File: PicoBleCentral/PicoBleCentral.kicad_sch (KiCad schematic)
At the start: 25 parts, among them J1 Screw_Terminal_01x02, J2 3V3 Sel, J3 keypad, J4 grove 2mm, J5 i2c, Q1 DMG2305UX-7, SW1 SW_Push, U1 AP7384-50Y, U2 Pico_RaspberryPico, U3 MCP23008-xSO, U4 AMS1117-3.3

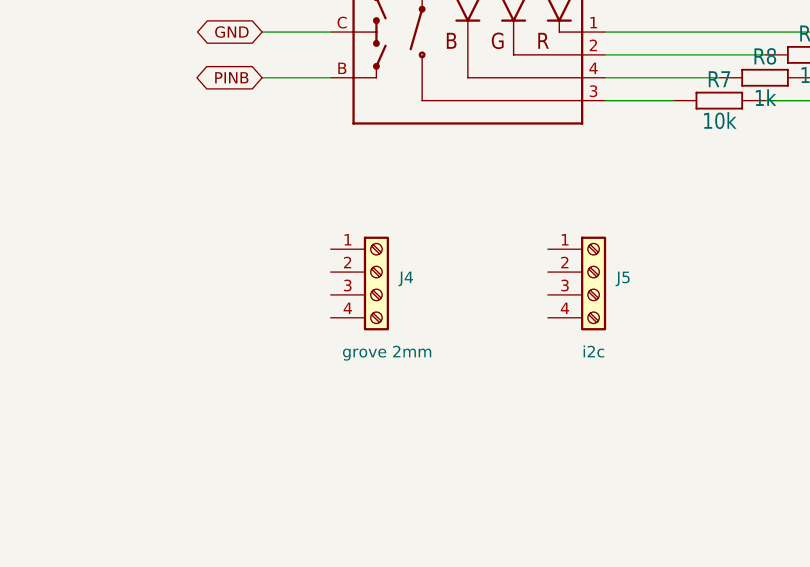
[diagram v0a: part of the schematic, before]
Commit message: 27/05/25 09:08 Arrakis.local
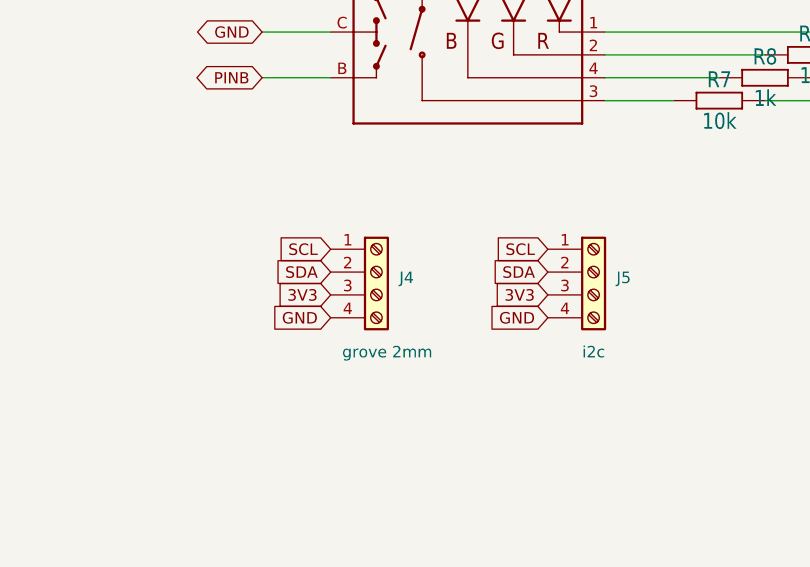
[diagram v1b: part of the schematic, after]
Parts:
- J4, J5: footprint (none) -> Seed Grove etc:HW4-SMD-2.0
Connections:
- net 3V3: now also J4.3 (Pin_3), J5.3 (Pin_3)
- net GND: now also J4.4 (Pin_4), J5.4 (Pin_4)
- net SCL: now also J4.1 (Pin_1), J5.1 (Pin_1)
- net SDA: now also J4.2 (Pin_2), J5.2 (Pin_2)
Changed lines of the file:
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@@
+    )
+  )
+  (global_label "3V3" (shape input) (at 218.44 127 180) (fields_autoplaced)
+    (effects (font (size 1.27 1.27)) (justify right))
+    (property "Intersheetrefs" "${INTERSHEET_REFS}" (at 212.0266 127 0)
+      (effects (font (size 1.27 1.27)) (justify right) hide)
     )
   )
@@
     (effects (font (size 1.27 1.27)) (justify right))
     (property "Intersheetrefs" "${INTERSHEET_REFS}" (at 170.0372 40.64 0)
+      (effects (font (size 1.27 1.27)) (justify right) hide)
+    )
+  )
+  (global_label "SCL" (shape input) (at 194.31 121.92 180) (fields_autoplaced)
+    (effects (font (size 1.27 1.27)) (justify right))
+    (property "Intersheetrefs" "${INTERSHEET_REFS}" (at 187.8966 121.92 0)
       (effects (font (size 1.27 1.27)) (justify right) hide)
     )
@@
     )
   )
+  (global_label "3V3" (shape input) (at 194.31 127 180) (fields_autoplaced)
+    (effects (font (size 1.27 1.27)) (justify right))
+    (property "Intersheetrefs" "${INTERSHEET_REFS}" (at 187.8966 127 0)
+      (effects (font (size 1.27 1.27)) (justify right) hide)
+    )
+  )
   (global_label "+5V" (shape input) (at 128.27 36.83 180) (fields_autoplaced)
     (effects (font (size 1.27 1.27)) (justify right))
@@
     )
   )
+  (global_label "SDA" (shape input) (at 194.31 124.46 180) (fields_autoplaced)
+    (effects (font (size 1.27 1.27)) (justify right))
+    (property "Intersheetrefs" "${INTERSHEET_REFS}" (at 187.8361 124.46 0)
+      (effects (font (size 1.27 1.27)) (justify right) hide)
+    )
+  )
   (global_label "PINA" (shape input) (at 140.97 137.16 0) (fields_autoplaced)
     (effects (font (size 1.27 1.27)) (justify left))
@@
     )
   )
+  (global_label "GND" (shape input) (at 218.44 129.54 180) (fields_autoplaced)
+    (effects (font (size 1.27 1.27)) (justify right))
+    (property "Intersheetrefs" "${INTERSHEET_REFS}" (at 211.6637 129.54 0)
+      (effects (font (size 1.27 1.27)) (justify right) hide)
+    )
+  )
   (global_label "RUN" (shape input) (at 82.55 147.32 0) (fields_autoplaced)
     (effects (font (size 1.27 1.27)) (justify left))
@@
     )
   )
+  (global_label "SDA" (shape input) (at 218.44 124.46 180) (fields_autoplaced)
+    (effects (font (size 1.27 1.27)) (justify right))
+    (property "Intersheetrefs" "${INTERSHEET_REFS}" (at 211.9661 124.46 0)
+      (effects (font (size 1.27 1.27)) (justify right) hide)
+    )
+  )
+  (global_label "SCL" (shape input) (at 218.44 121.92 180) (fields_autoplaced)
+    (effects (font (size 1.27 1.27)) (justify right))
+    (property "Intersheetrefs" "${INTERSHEET_REFS}" (at 212.0266 121.92 0)
+      (effects (font (size 1.27 1.27)) (justify right) hide)
+    )
+  )
   (global_label "3V3_OUT" (shape input) (at 161.29 72.39 0) (fields_autoplaced)
     (effects (font (size 1.27 1.27)) (justify left))
     (property "Intersheetrefs" "${INTERSHEET_REFS}" (at 172.379 72.39 0)
       (effects (font (size 1.27 1.27)) (justify left) hide)
+    )
+  )
+  (global_label "GND" (shape input) (at 194.31 129.54 180) (fields_autoplaced)
+    (effects (font (size 1.27 1.27)) (justify right))
+    (property "Intersheetrefs" "${INTERSHEET_REFS}" (at 187.5337 129.54 0)
+      (effects (font (size 1.27 1.27)) (justify right) hide)
     )
   )
@@
       (effects (font (size 1.27 1.27)) (justify left))
     )
-    (property "Footprint" "" (at 199.39 124.46 0)
+    (property "Footprint" "Seed Grove etc:HW4-SMD-2.0" (at 199.39 124.46 0)
       (effects (font (size 1.27 1.27)) hide)
     )
@@
       (effects (font (size 1.27 1.27)) (justify left))
     )
-    (property "Footprint" "" (at 223.52 124.46 0)
-      (effects (font (size 1.27 1.27)) hide)
-    )
+    (property "Footprint" "Seed Grove etc:HW4-SMD-2.0" (at 223.52 124.46 0)
+      (effects (font (size 1.27 1.27)) hide)
+    )
